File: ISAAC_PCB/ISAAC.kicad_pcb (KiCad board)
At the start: 2 copper layers, 49 parts, among them J1 Conn_02x04_Top_Bottom, J2 Conn_02x04_Top_Bottom, J3 Screw_Terminal_01x02, J4 XT60PW-M, U10 DMN4026SSD, U11 LM337_TO3, U2 DMN4026SSD, U3 DMN4026SSD, U4 DMN4026SSD, U5 DMN4026SSD, U6 module_mpu6050, U7 DMN4026SSD, U8 DMN4026SSD, U9 DMN4026SSD

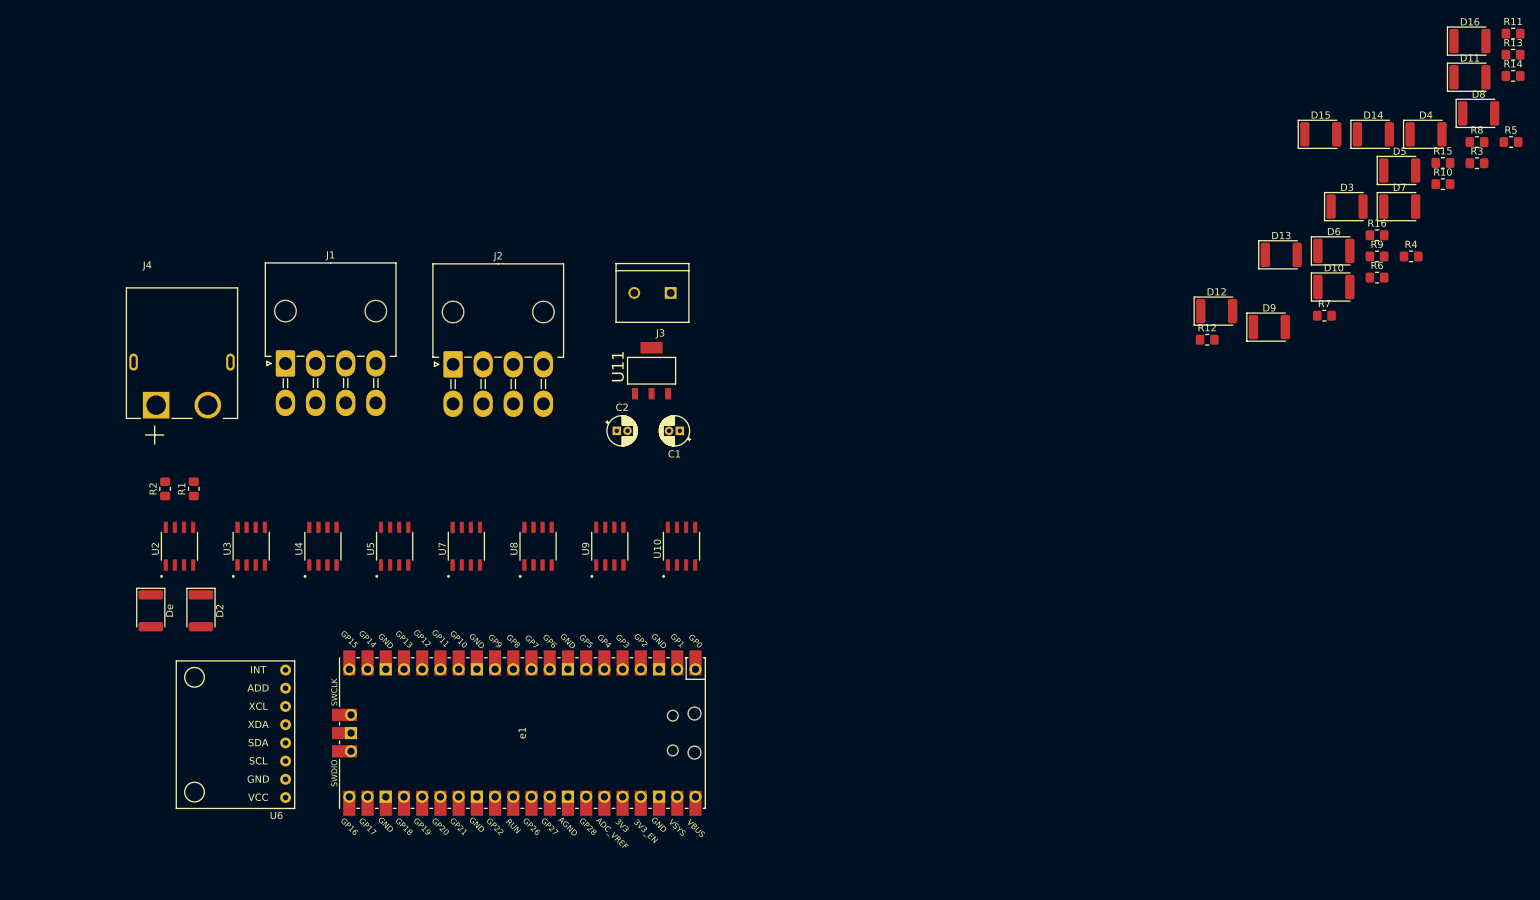
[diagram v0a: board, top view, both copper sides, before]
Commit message: Finished Version 1
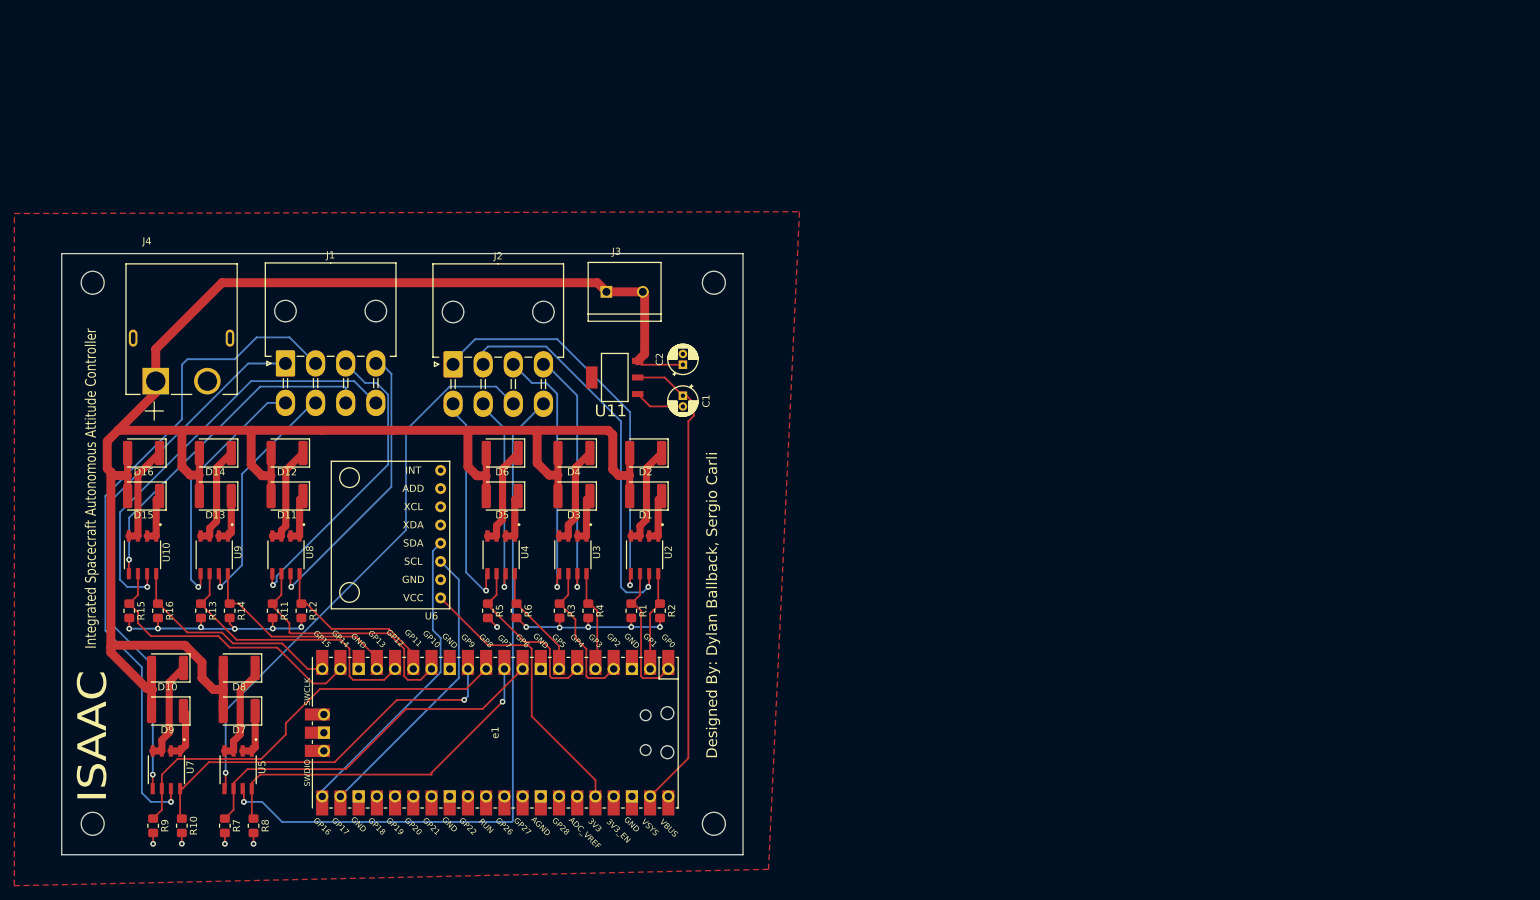
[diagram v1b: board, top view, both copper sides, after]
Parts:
- added H1: MountingHole, MountingHole:MountingHole_3.2mm_M3, F.Cu at (72.9, 123.7)
- added H2: MountingHole, MountingHole:MountingHole_3.2mm_M3, F.Cu at (159.5, 48.3)
- added H3: MountingHole, MountingHole:MountingHole_3.2mm_M3, F.Cu at (72.9, 48.3)
- added H4: MountingHole, MountingHole:MountingHole_3.2mm_M3, F.Cu at (159.5, 123.7)
- moved R13 198.7 mm to (88.0, 94.0), turned to 270 degrees
- moved R10 197.3 mm to (85.3, 124.0), turned to 270 degrees
- moved R8 195.4 mm to (95.3, 124.0), turned to 270 degrees
- moved R14 193.9 mm to (92.0, 94.0), turned to 270 degrees
- moved D16 193.6 mm to (80.0, 72.0), turned to 180 degrees
- moved R15 193.5 mm to (78.0, 94.0), turned to 270 degrees
- moved R11 190.8 mm to (98.0, 94.0), turned to 270 degrees
- moved D8 189.3 mm to (93.3, 102.0), turned to 180 degrees
- moved R9 188.2 mm to (81.3, 124.0), turned to 270 degrees
- moved R16 177.9 mm to (82.0, 94.0), turned to 270 degrees
- moved D7 176.4 mm to (93.3, 108.0), turned to 180 degrees
- moved D11 175.0 mm to (100.0, 78.0), turned to 180 degrees
- moved D15 171.7 mm to (80.0, 78.0), turned to 180 degrees
- moved D10 171.1 mm to (83.3, 102.0), turned to 180 degrees
- moved R7 169.0 mm to (91.3, 124.0), turned to 270 degrees
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- renumbered De to D1
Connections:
- C2 pad 1: +BATT -> VCC
- D12 pad 2: Net-(D12-Pad2) -> VCC
- J3 pad 1: +BATT -> VCC
- J3 pad 2: +BATT -> VCC
- J4 pad 1: +BATT -> VCC
- U11 pad 3: +BATT -> VCC
- U8 pad 3: Net-(U8-Pad3) -> Net-(D12-Pad1)
- U8 pad 4: Net-(U8-Pad3) -> Net-(D12-Pad1)
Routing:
- net VCC: track 0.00 -> 321.3 mm
- net SOL8: track 0.00 -> 100.6 mm, vias 0 -> 1
- net SOL10: track 0.00 -> 94.5 mm, vias 0 -> 1
- net SOL7: track 0.00 -> 78.9 mm, vias 0 -> 1
- net SOL9: track 0.00 -> 74.8 mm, vias 0 -> 1
- net GND: track 0.00 -> 74.3 mm, vias 0 -> 16
- net +3.3VA: track 0.00 -> 66.7 mm
- net SOL16: track 0.00 -> 60.0 mm, vias 0 -> 1
- net GATE9: track 0.00 -> 58.9 mm
- net SOL1: track 0.00 -> 56.4 mm, vias 0 -> 1
- net SOL2: track 0.00 -> 55.1 mm, vias 0 -> 1
- net GATE10: track 0.00 -> 53.6 mm, vias 0 -> 1
- net GATE7: track 0.00 -> 52.3 mm
- net GATE8: track 0.00 -> 49.6 mm, vias 0 -> 1
- net SOL15: track 0.00 -> 48.0 mm, vias 0 -> 1
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- added copper zone on F.Cu, net GND
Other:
- board outline added: 95 x 83.8 mm
- board text added: "Designed By: Dylan Ballback, Sergio Carli"
- board text added: "ISAAC"
- board text added: "Integrated Spacecraft Autonomous Attitude Controller"
